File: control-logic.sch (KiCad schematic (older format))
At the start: 34 parts, among them U2 STM32F072R, U3 MCP2562, X1 8.000 MHz

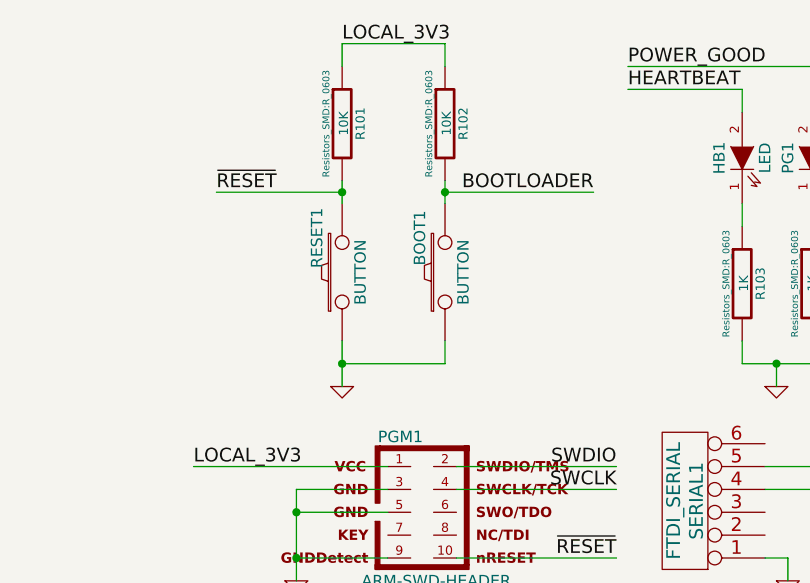
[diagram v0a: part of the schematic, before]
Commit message: Latest changes (so old I don't remember)
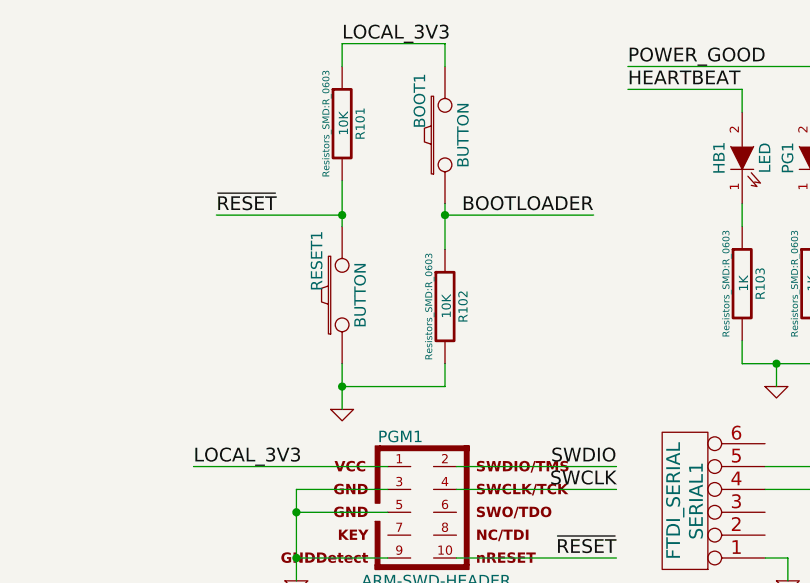
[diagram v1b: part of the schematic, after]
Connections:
- net BOOTLOADER: now also BOOT1.1, R102.1; no longer BOOT1.2, R102.2
- net CONTROL_3V3: now also BOOT1.2; no longer R102.1
- net GND: now also R102.2; no longer BOOT1.1
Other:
- moved on the sheet: BOOT1, R102, RESET1
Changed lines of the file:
@@
 $EndComp
 $Comp
-L GND-RESCUE-base-module-hardware-v2 #PWR027
+L GND-RESCUE-base-module-hardware-v2 #PWR028
 U 1 1 5325BA22
 P 9050 6650
-F 0 "#PWR027" H 9050 6650 30  0001 C CNN
+F 0 "#PWR028" H 9050 6650 30  0001 C CNN
 F 1 "GND" H 9050 6580 30  0001 C CNN
 F 2 "" H 9050 6650 60  0000 C CNN
@@
 VSOL_PRECHARGE_PWM
 $Comp
-L GND-RESCUE-base-module-hardware-v2 #PWR028
+L GND-RESCUE-base-module-hardware-v2 #PWR029
 U 1 1 53262BD9
 P 3050 5600
-F 0 "#PWR028" H 3050 5600 30  0001 C CNN
+F 0 "#PWR029" H 3050 5600 30  0001 C CNN
 F 1 "GND" H 3050 5530 30  0001 C CNN
 F 2 "" H 3050 5600 60  0000 C CNN
@@
 $EndComp
 $Comp
-L GND-RESCUE-base-module-hardware-v2 #PWR029
+L GND-RESCUE-base-module-hardware-v2 #PWR030
 U 1 1 53264B7B
 P 1200 2100
-F 0 "#PWR029" H 1200 2100 30  0001 C CNN
+F 0 "#PWR030" H 1200 2100 30  0001 C CNN
 F 1 "GND" H 1200 2030 30  0001 C CNN
 F 2 "" H 1200 2100 60  0000 C CNN
@@
 L SW_PUSH RESET1
 U 1 1 53267B06
-P 8050 1750
-F 0 "RESET1" H 8200 1860 50  0000 C CNN
-F 1 "BUTTON" H 8050 1670 50  0000 C CNN
-F 2 "Buttons_Switches_ThroughHole:SW_PUSH_SMALL" H 8050 1750 60  0001 C CNN
-F 3 "~" H 8050 1750 60  0000 C CNN
-	1    8050 1750
+P 8050 1850
+F 0 "RESET1" H 8200 1960 50  0000 C CNN
+F 1 "BUTTON" H 8050 1770 50  0000 C CNN
+F 2 "Buttons_Switches_ThroughHole:SW_PUSH_SMALL" H 8050 1850 60  0001 C CNN
+F 3 "~" H 8050 1850 60  0000 C CNN
+	1    8050 1850
 	0    -1   -1   0
 $EndComp
@@
 L SW_PUSH BOOT1
 U 1 1 53267B15
-P 8500 1750
-F 0 "BOOT1" H 8650 1860 50  0000 C CNN
-F 1 "BUTTON" H 8500 1670 50  0000 C CNN
-F 2 "Buttons_Switches_ThroughHole:SW_PUSH_SMALL" H 8500 1750 60  0001 C CNN
-F 3 "~" H 8500 1750 60  0000 C CNN
-	1    8500 1750
+P 8500 1150
+F 0 "BOOT1" H 8650 1260 50  0000 C CNN
+F 1 "BUTTON" H 8500 1070 50  0000 C CNN
+F 2 "Buttons_Switches_ThroughHole:SW_PUSH_SMALL" H 8500 1150 60  0001 C CNN
+F 3 "~" H 8500 1150 60  0000 C CNN
+	1    8500 1150
 	0    -1   -1   0
 $EndComp
@@
 L R-RESCUE-base-module-hardware-v2 R102
 U 1 1 53267B42
-P 8500 1100
-F 0 "R102" V 8580 1100 40  0000 C CNN
-F 1 "10K" V 8507 1101 40  0000 C CNN
-F 2 "Resistors_SMD:R_0603" V 8430 1100 30  0000 C CNN
-F 3 "~" H 8500 1100 30  0000 C CNN
-	1    8500 1100
+P 8500 1900
+F 0 "R102" V 8580 1900 40  0000 C CNN
+F 1 "10K" V 8507 1901 40  0000 C CNN
+F 2 "Resistors_SMD:R_0603" V 8430 1900 30  0000 C CNN
+F 3 "~" H 8500 1900 30  0000 C CNN
+	1    8500 1900
 	1    0    0    -1
 $EndComp
@@
 $EndComp
 $Comp
-L GND-RESCUE-base-module-hardware-v2 #PWR030
+L GND-RESCUE-base-module-hardware-v2 #PWR031
 U 1 1 53268402
 P 6350 6550
-F 0 "#PWR030" H 6350 6550 30  0001 C CNN
+F 0 "#PWR031" H 6350 6550 30  0001 C CNN
 F 1 "GND" H 6350 6480 30  0001 C CNN
 F 2 "" H 6350 6550 60  0000 C CNN
@@
 Text Label 6350 5850 0    60   ~ 0
 LOCAL_3V3
-Text Label 9150 1400 2    60   ~ 0
+Text Label 9150 1500 2    60   ~ 0
 BOOTLOADER
-Text Label 7500 1400 0    60   ~ 0
+Text Label 7500 1500 0    60   ~ 0
 ~RESET
 Text Label 8050 750  0    60   ~ 0
 LOCAL_3V3
 $Comp
-L GND-RESCUE-base-module-hardware-v2 #PWR031
+L GND-RESCUE-base-module-hardware-v2 #PWR032
 U 1 1 53268FE5
-P 8050 2250
-F 0 "#PWR031" H 8050 2250 30  0001 C CNN
-F 1 "GND" H 8050 2180 30  0001 C CNN
-F 2 "" H 8050 2250 60  0000 C CNN
-F 3 "" H 8050 2250 60  0000 C CNN
-	1    8050 2250
-	1    0    0    -1
-$EndComp
-$Comp
-L GND-RESCUE-base-module-hardware-v2 #PWR032
+P 8050 2350
+F 0 "#PWR032" H 8050 2350 30  0001 C CNN
+F 1 "GND" H 8050 2280 30  0001 C CNN
+F 2 "" H 8050 2350 60  0000 C CNN
+F 3 "" H 8050 2350 60  0000 C CNN
+	1    8050 2350
+	1    0    0    -1
+$EndComp
+$Comp
+L GND-RESCUE-base-module-hardware-v2 #PWR033
 U 1 1 532697A4
 P 9950 2250
-F 0 "#PWR032" H 9950 2250 30  0001 C CNN
+F 0 "#PWR033" H 9950 2250 30  0001 C CNN
 F 1 "GND" H 9950 2180 30  0001 C CNN
 F 2 "" H 9950 2250 60  0000 C CNN
@@
 POWER_GOOD
 $Comp
-L GND-RESCUE-base-module-hardware-v2 #PWR033
+L GND-RESCUE-base-module-hardware-v2 #PWR034
 U 1 1 5326A151
 P 7850 3100
-F 0 "#PWR033" H 7850 3100 30  0001 C CNN
+F 0 "#PWR034" H 7850 3100 30  0001 C CNN
 F 1 "GND" H 7850 3030 30  0001 C CNN
 F 2 "" H 7850 3100 60  0000 C CNN
@@
 TXD
 $Comp
-L GND-RESCUE-base-module-hardware-v2 #PWR034
+L GND-RESCUE-base-module-hardware-v2 #PWR035
 U 1 1 5326B790
 P 10000 3100
-F 0 "#PWR034" H 10000 3100 30  0001 C CNN
+F 0 "#PWR035" H 10000 3100 30  0001 C CNN
 F 1 "GND" H 10000 3030 30  0001 C CNN
 F 2 "" H 10000 3100 60  0000 C CNN
@@
 SDA
 $Comp
-L GND-RESCUE-base-module-hardware-v2 #PWR035
+L GND-RESCUE-base-module-hardware-v2 #PWR036
 U 1 1 533CA56F
 P 9100 4150
-F 0 "#PWR035" H 9100 4150 30  0001 C CNN
+F 0 "#PWR036" H 9100 4150 30  0001 C CNN
 F 1 "GND" H 9100 4080 30  0001 C CNN
 F 2 "" H 9100 4150 60  0000 C CNN
@@
 $EndComp
 $Comp
-L GND-RESCUE-base-module-hardware-v2 #PWR036
+L GND-RESCUE-base-module-hardware-v2 #PWR037
 U 1 1 54EC01AF
 P 2200 7650
-F 0 "#PWR036" H 2200 7650 30  0001 C CNN
+F 0 "#PWR037" H 2200 7650 30  0001 C CNN
 F 1 "GND" H 2200 7580 30  0001 C CNN
 F 2 "" H 2200 7650 60  0000 C CNN
@@
 $EndComp
 $Comp
-L GND-RESCUE-base-module-hardware-v2 #PWR037
+L GND-RESCUE-base-module-hardware-v2 #PWR038
 U 1 1 54EC1E75
 P 3900 7650
-F 0 "#PWR037" H 3900 7650 30  0001 C CNN
+F 0 "#PWR038" H 3900 7650 30  0001 C CNN
 F 1 "GND" H 3900 7580 30  0001 C CNN
 F 2 "" H 3900 7650 60  0000 C CNN
@@
 	8500 750  8500 850
 Wire Wire Line
-	8050 1350 8050 1450
-Wire Wire Line
-	8500 1350 8500 1450
-Wire Wire Line
-	8050 2050 8050 2250
-Wire Wire Line
-	8050 2150 8500 2150
-Wire Wire Line
-	8500 2150 8500 2050
-Wire Wire Line
-	9150 1400 8500 1400
-Connection ~ 8500 1400
-Wire Wire Line
-	7500 1400 8050 1400
-Connection ~ 8050 1400
-Connection ~ 8050 2150
+	8050 1350 8050 1550
+Wire Wire Line
+	8500 1450 8500 1650
+Wire Wire Line
+	8050 2150 8050 2350
+Wire Wire Line
+	8050 2250 8500 2250
+Wire Wire Line
+	8500 2250 8500 2150
+Wire Wire Line
+	9150 1500 8500 1500
+Connection ~ 8500 1500
+Wire Wire Line
+	7500 1500 8050 1500
+Connection ~ 8050 1500
+Connection ~ 8050 2250
 Wire Wire Line
 	9800 1450 9800 1550
